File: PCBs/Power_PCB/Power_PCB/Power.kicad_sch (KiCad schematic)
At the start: 19 parts, among them J1 Conn_01x02, J12 Conn_01x04, J2 Conn_01x02, J3 Conn_01x02, Q1 SUD45P03-09, SW1 SW_Push_Open, U2 AMS1117-3.3, U5 TVS3300DRV

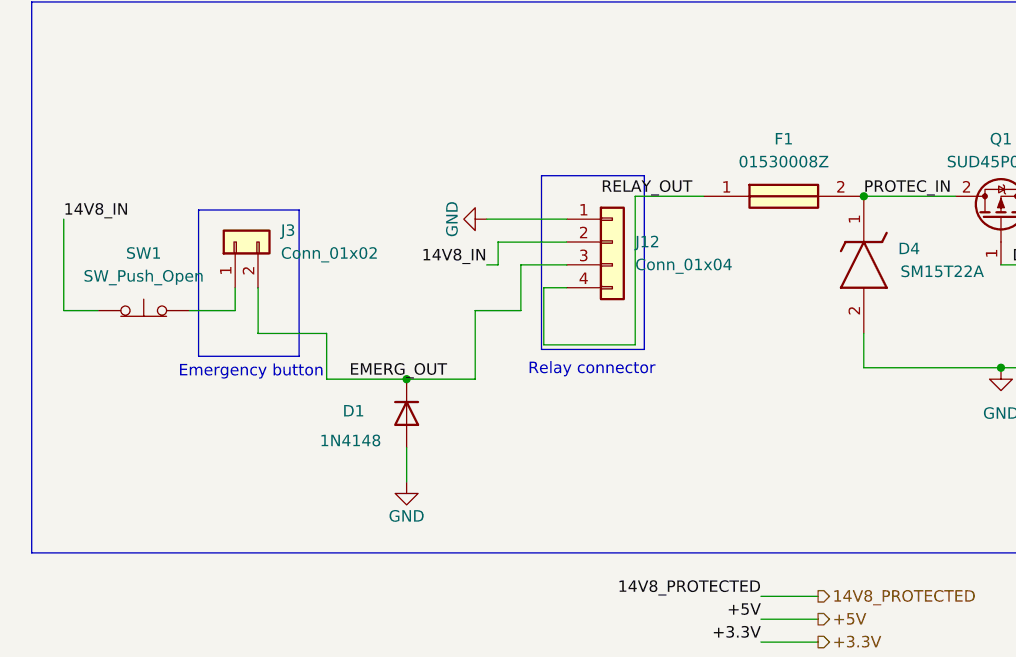
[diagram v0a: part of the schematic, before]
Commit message: Second iteration power board
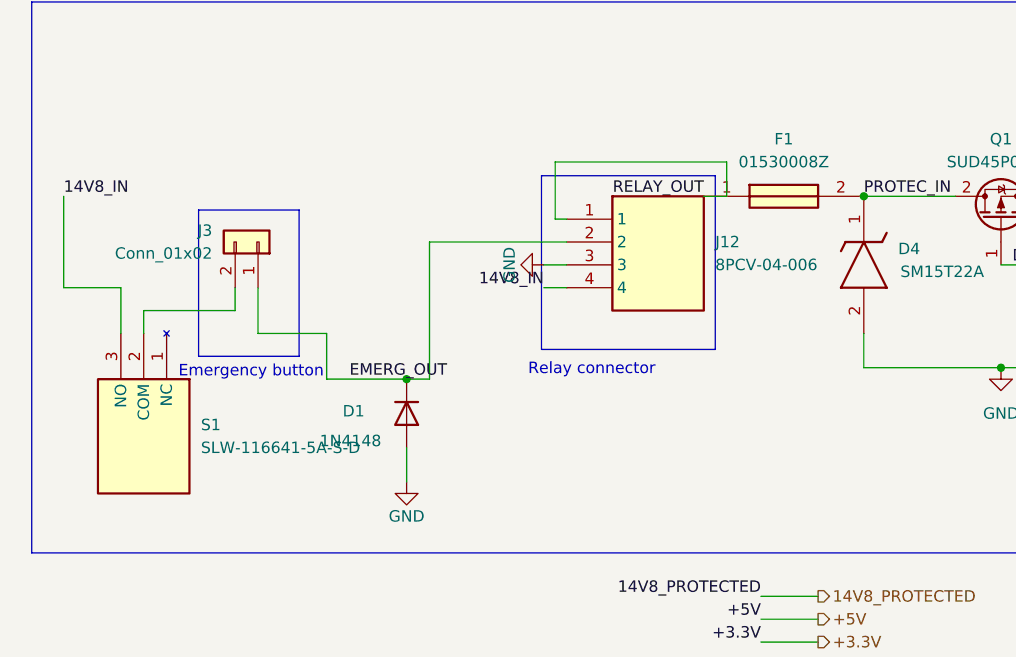
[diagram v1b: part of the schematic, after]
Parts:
- removed J12: Conn_01x04, TerminalBlock:TerminalBlock_Altech_AK300-4_P5.00mm, symbol Connector_Generic:Conn_01x04
- removed SW1: SW_Push_Open, Button_Switch_THT:SW_Slide_SPDT_Straight_CK_OS102011MS2Q, symbol Switch:SW_Push_Open
- added J12: 8PCV-04-006, SHDR4W114P0X1112_1X4_4628X2032X1956P, symbol 8PCV-04-006:8PCV-04-006
- added S1: SLW-116641-5A-S-D, SLW1166415ASD, symbol SLW-116641-5A-S-D:SLW-116641-5A-S-D
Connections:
- net 14V8_IN: now also J12.4, S1.3 (NO)
- net EMERG_OUT: now also J3.1 (Pin_1), J12.2; no longer J3.2 (Pin_2)
- net GND: now also J12.3
- net RELAY_OUT: now also J12.1
- new net: J3.2 (Pin_2), S1.2 (COM)
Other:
- moved on the sheet: J3

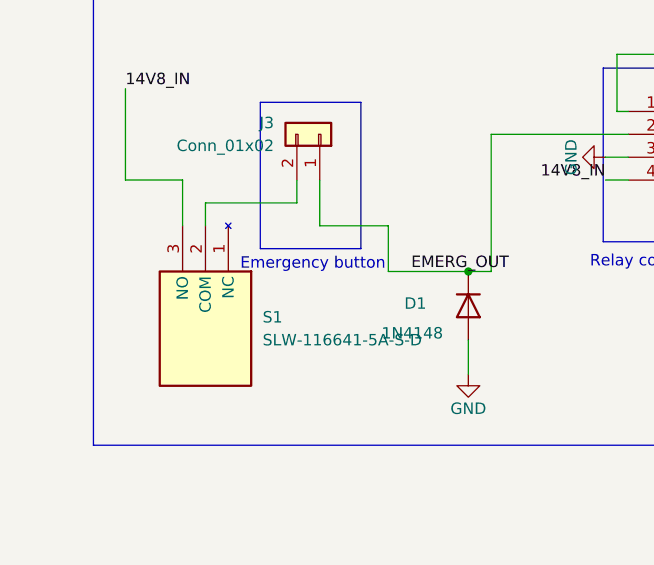
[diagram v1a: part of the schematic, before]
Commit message: Power board revisions
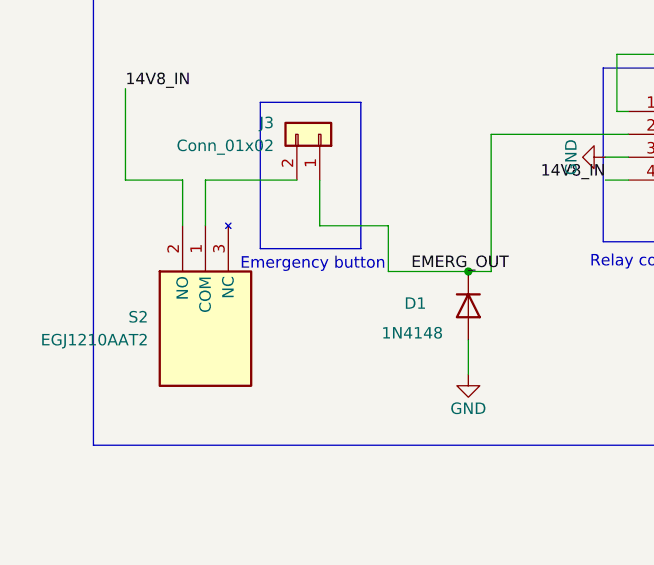
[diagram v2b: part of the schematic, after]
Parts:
- removed S1: SLW-116641-5A-S-D, SLW1166415ASD, symbol SLW-116641-5A-S-D:SLW-116641-5A-S-D
- added S2: EGJ1210AAT2, EGJ1210AAT2, symbol EGJ1210AAT2:EGJ1210AAT2
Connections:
- net 14V8_IN: now also S2.2 (NO)
- net at J3.2 (Pin_2): now also S2.1 (COM)
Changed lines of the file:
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@@
 	(wire
 		(pts
-			(xy 88.9 110.49) (xy 99.06 110.49)
+			(xy 88.9 107.95) (xy 99.06 107.95)
 		)
 		(stroke
@@
 	(wire
 		(pts
-			(xy 204.47 50.8) (xy 220.98 50.8)
+			(xy 88.9 107.95) (xy 88.9 113.03)
 		)
 		(stroke
@@
 	(wire
 		(pts
-			(xy 88.9 110.49) (xy 88.9 113.03)
+			(xy 204.47 50.8) (xy 220.98 50.8)
 		)
 		(stroke
@@
 		(pts
 			(xy 153.67 97.79) (xy 151.13 97.79)
-		)
-		(stroke
-			(width 0)
-			(type default)
-		)
-	)
-	(wire
-		(pts
-			(xy 99.06 107.95) (xy 99.06 110.49)
 		)
 		(stroke
@@
 	)
 	(symbol
-		(lib_id "SLW-116641-5A-S-D:SLW-116641-5A-S-D")
-		(at 91.44 113.03 270)
-		(unit 1)
-		(exclude_from_sim no)
-		(in_bom yes)
-		(on_board yes)
-		(dnp no)
-		(fields_autoplaced yes)
-		(property "Reference" "S1"
-			(at 95.25 123.1899 90)
-			(effects
-				(font
-					(size 1.27 1.27)
-				)
-				(justify left)
-			)
-		)
-		(property "Value" "SLW-116641-5A-S-D"
-			(at 95.25 125.7299 90)
-			(effects
-				(font
-					(size 1.27 1.27)
-				)
-				(justify left)
-			)
-		)
-		(property "Footprint" "SLW1166415ASD"
-			(at -3.48 132.08 0)
-			(effects
-				(font
-					(size 1.27 1.27)
-				)
-				(justify left top)
-				(hide yes)
-			)
-		)
-		(property "Datasheet" "https://www.sameskydevices.com/product/resource/supplyframepdf/slw-116641-5a-s-d.pdf"
-			(at -103.48 132.08 0)
-			(effects
-				(font
-					(size 1.27 1.27)
-				)
-				(justify left top)
-				(hide yes)
-			)
-		)
-		(property "Description" "11.6 x 6 x 4.1 mm, 5 mm Raised Slide Actuator, Through Hole, Slide Switch"
-			(at 91.44 113.03 0)
-			(effects
-				(font
-					(size 1.27 1.27)
-				)
-				(hide yes)
-			)
-		)
-		(property "Height" "11.3"
-			(at -303.48 132.08 0)
-			(effects
-				(font
-					(size 1.27 1.27)
-				)
-				(justify left top)
-				(hide yes)
-			)
-		)
-		(property "Manufacturer_Name" "Same Sky"
-			(at -403.48 132.08 0)
-			(effects
-				(font
-					(size 1.27 1.27)
-				)
-				(justify left top)
-				(hide yes)
-			)
-		)
-		(property "Manufacturer_Part_Number" "SLW-116641-5A-S-D"
-			(at -503.48 132.08 0)
-			(effects
-				(font
-					(size 1.27 1.27)
-				)
-				(justify left top)
-				(hide yes)
-			)
-		)
-		(property "Mouser Part Number" "179-SLW1166415ASD"
-			(at -603.48 132.08 0)
-			(effects
-				(font
-					(size 1.27 1.27)
-				)
-				(justify left top)
-				(hide yes)
-			)
-		)
-		(property "Mouser Price/Stock" "https://www.mouser.co.uk/ProductDetail/Same-Sky/SLW-116641-5A-S-D?qs=IKkN%2F947nfBZSdW8n5Vqgw%3D%3D"
-			(at -703.48 132.08 0)
-			(effects
-				(font
-					(size 1.27 1.27)
-				)
-				(justify left top)
-				(hide yes)
-			)
-		)
-		(property "Arrow Part Number" "SLW-116641-5A-S-D"
-			(at -803.48 132.08 0)
-			(effects
-				(font
-					(size 1.27 1.27)
-				)
-				(justify left top)
-				(hide yes)
-			)
-		)
-		(property "Arrow Price/Stock" "https://www.arrow.com/en/products/slw-116641-5a-s-d/cui-devices?utm_currency=USD&region=nac"
-			(at -903.48 132.08 0)
-			(effects
-				(font
-					(size 1.27 1.27)
-				)
-				(justify left top)
-				(hide yes)
-			)
-		)
-		(pin "1"
-		)
-		(pin "3"
-		)
-		(pin "2"
-		)
-		(instances
-			(project ""
-				(path "/87325cad-d0d9-4e34-97c3-9178133a19b1/ceb728e0-0a2f-47f1-b8f2-8a2cf5487bda"
-					(reference "S1")
-					(unit 1)
-				)
-			)
-		)
-	)
-	(symbol
 		(lib_id "Diode:1N4148")
 		(at 118.11 121.92 270)
@@
 					(unit 1)
 				)
+			)
+		)
+	)
+	(symbol
+		(lib_id "EGJ1210AAT2:EGJ1210AAT2")
+		(at 86.36 113.03 90)
+		(mirror x)
+		(unit 1)
+		(exclude_from_sim no)
+		(in_bom yes)
+		(on_board yes)
+		(dnp no)
+		(property "Reference" "S2"
+			(at 82.55 123.1899 90)
+			(effects
+				(font
+					(size 1.27 1.27)
+				)
+				(justify left)
+			)
+		)
+		(property "Value" "EGJ1210AAT2"
+			(at 82.55 125.7299 90)
+			(effects
+				(font
+					(size 1.27 1.27)
+				)
+				(justify left)
+			)
+		)
+		(property "Footprint" "EGJ1210AAT2"
+			(at 181.28 132.08 0)
+			(effects
+				(font
+					(size 1.27 1.27)
+				)
+				(justify left top)
+				(hide yes)
+			)
+		)
+		(property "Datasheet" "https://configured-product-images.s3.amazonaws.com/2D/specs/EGJ1210AAT2.pdf"
+			(at 281.28 132.08 0)
+			(effects
+				(font
+					(size 1.27 1.27)
+				)
+				(justify left top)
+				(hide yes)
+			)
+		)
+		(property "Description" "SLIDE, 300mA / 500mA, 24VDC / 12VDC SPDT, On-On Through Hole, Right Angle"
+			(at 86.36 113.03 0)
+			(effects
+				(font
+					(size 1.27 1.27)
+				)
+				(hide yes)
+			)
+		)
+		(property "Height" "2.75"
+			(at 481.28 132.08 0)
+			(effects
+				(font
+					(size 1.27 1.27)
+				)
+				(justify left top)
+				(hide yes)
+			)
+		)
+		(property "Manufacturer_Name" "E-Switch"
+			(at 581.28 132.08 0)
+			(effects
+				(font
+					(size 1.27 1.27)
+				)
+				(justify left top)
+				(hide yes)
+			)
+		)
+		(property "Manufacturer_Part_Number" "EGJ1210AAT2"
+			(at 681.28 132.08 0)
+			(effects
+				(font
+					(size 1.27 1.27)
+				)
+				(justify left top)
+				(hide yes)
+			)
+		)
+		(property "Mouser Part Number" "612-EGJ1210AAT2"
+			(at 781.28 132.08 0)
+			(effects
+				(font
+					(size 1.27 1.27)
+				)
+				(justify left top)
+				(hide yes)
+			)
+		)
+		(property "Mouser Price/Stock" "https://www.mouser.co.uk/ProductDetail/E-Switch/EGJ1210AAT2?qs=%252BXxaIXUDbq28DPumZsnIIA%3D%3D"
+			(at 881.28 132.08 0)
+			(effects
+				(font
+					(size 1.27 1.27)
+				)
+				(justify left top)
+				(hide yes)
+			)
+		)
+		(property "Arrow Part Number" ""
+			(at 981.28 132.08 0)
+			(effects
+				(font
+					(size 1.27 1.27)
+				)
+				(justify left top)
+				(hide yes)
+			)
+		)
+		(property "Arrow Price/Stock" ""
+			(at 1081.28 132.08 0)
+			(effects
+				(font
+					(size 1.27 1.27)
+				)
+				(justify left top)
+				(hide yes)
+			)
+		)
+		(pin "1"
+		)
+		(pin "2"
+		)
+		(pin "3"
+		)
+		(instances
+			(project ""
+				(path "/87325cad-d0d9-4e34-97c3-9178133a19b1/ceb728e0-0a2f-47f1-b8f2-8a2cf5487bda"
+					(reference "S2")
+					(unit 1)
+				)

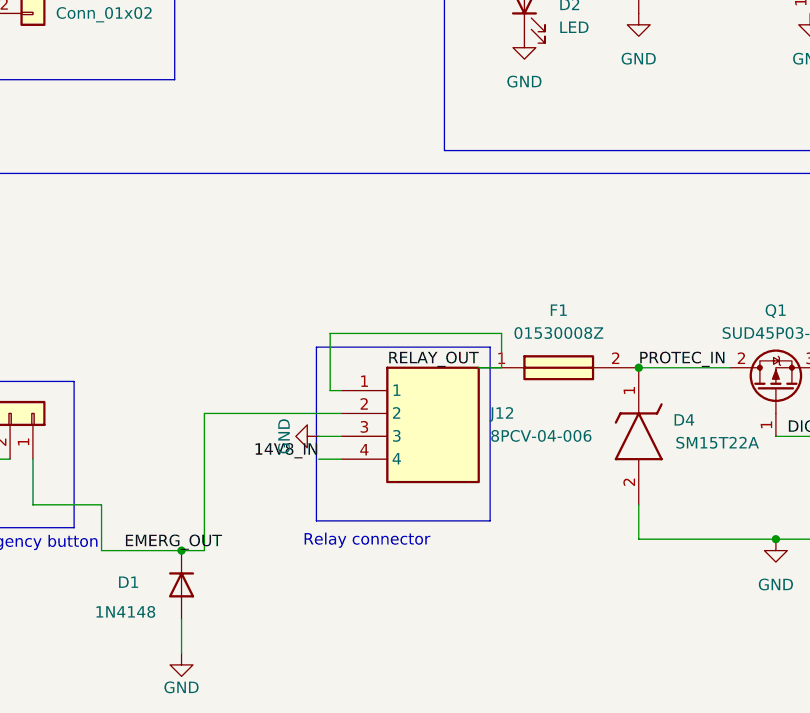
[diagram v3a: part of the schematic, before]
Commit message: follow up meeting changes
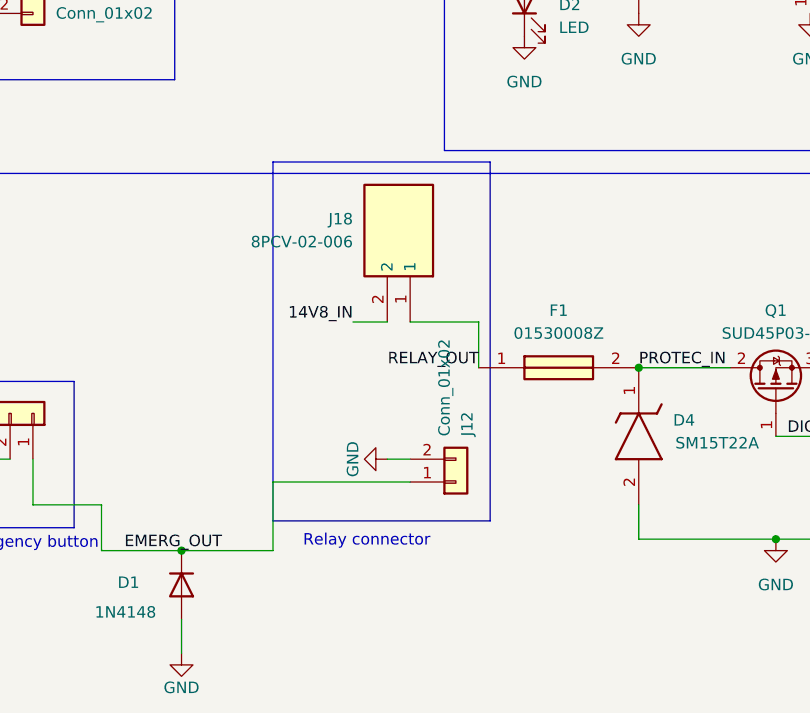
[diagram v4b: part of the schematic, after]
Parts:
- removed J12: 8PCV-04-006, SHDR4W114P0X1112_1X4_4628X2032X1956P, symbol 8PCV-04-006:8PCV-04-006
- added J12: Conn_01x02, TerminalBlock:TerminalBlock_Altech_AK300-2_P5.00mm, symbol Connector_Generic:Conn_01x02
- added J18: 8PCV-02-006, 8PCV02006, symbol 8PCV-02-006:8PCV-02-006
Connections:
- net 14V8_IN: now also J18.2
- net EMERG_OUT: now also J12.1 (Pin_1)
- net GND: now also J12.2 (Pin_2)
- net RELAY_OUT: now also J18.1
